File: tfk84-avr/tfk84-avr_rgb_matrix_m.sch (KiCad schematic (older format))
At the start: 42 parts

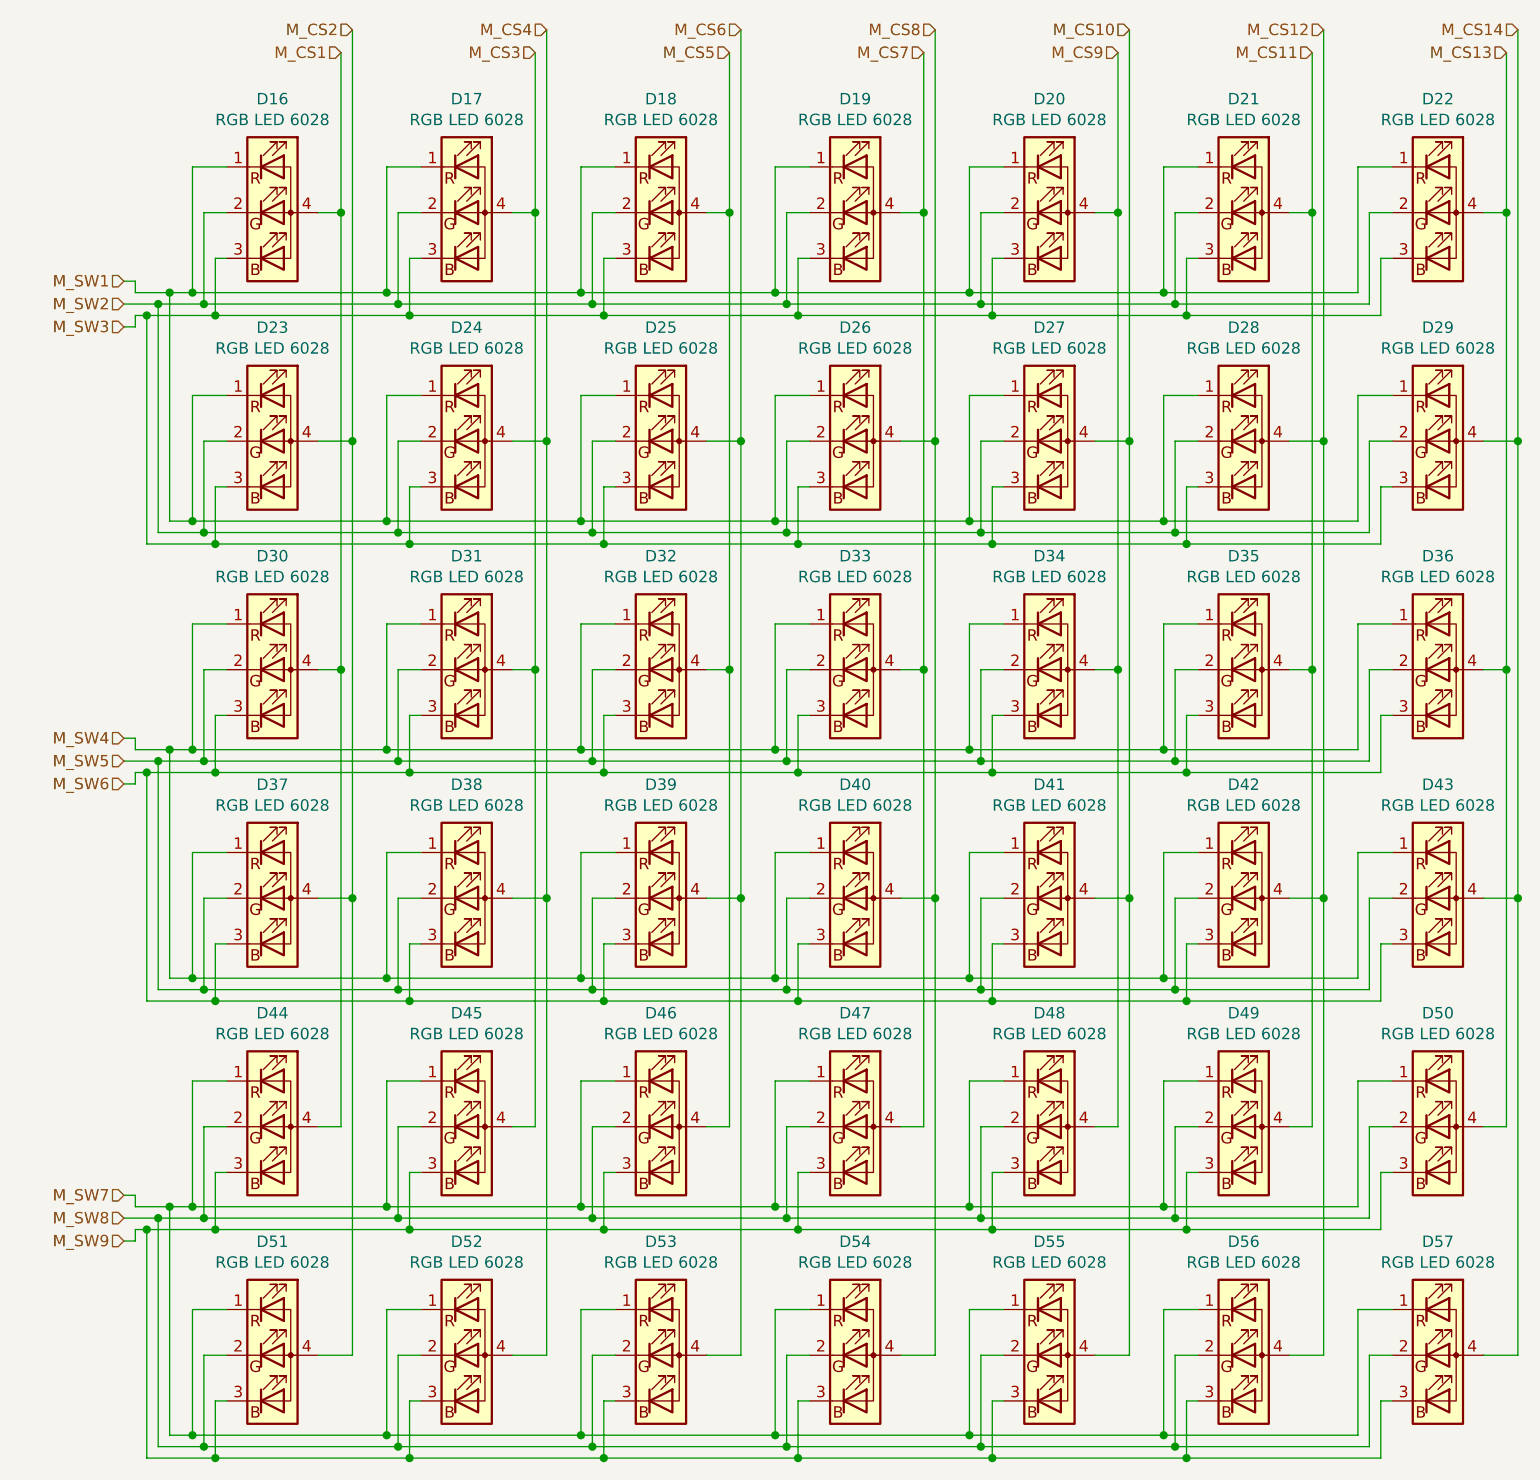
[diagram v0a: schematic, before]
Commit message: Begin PCB
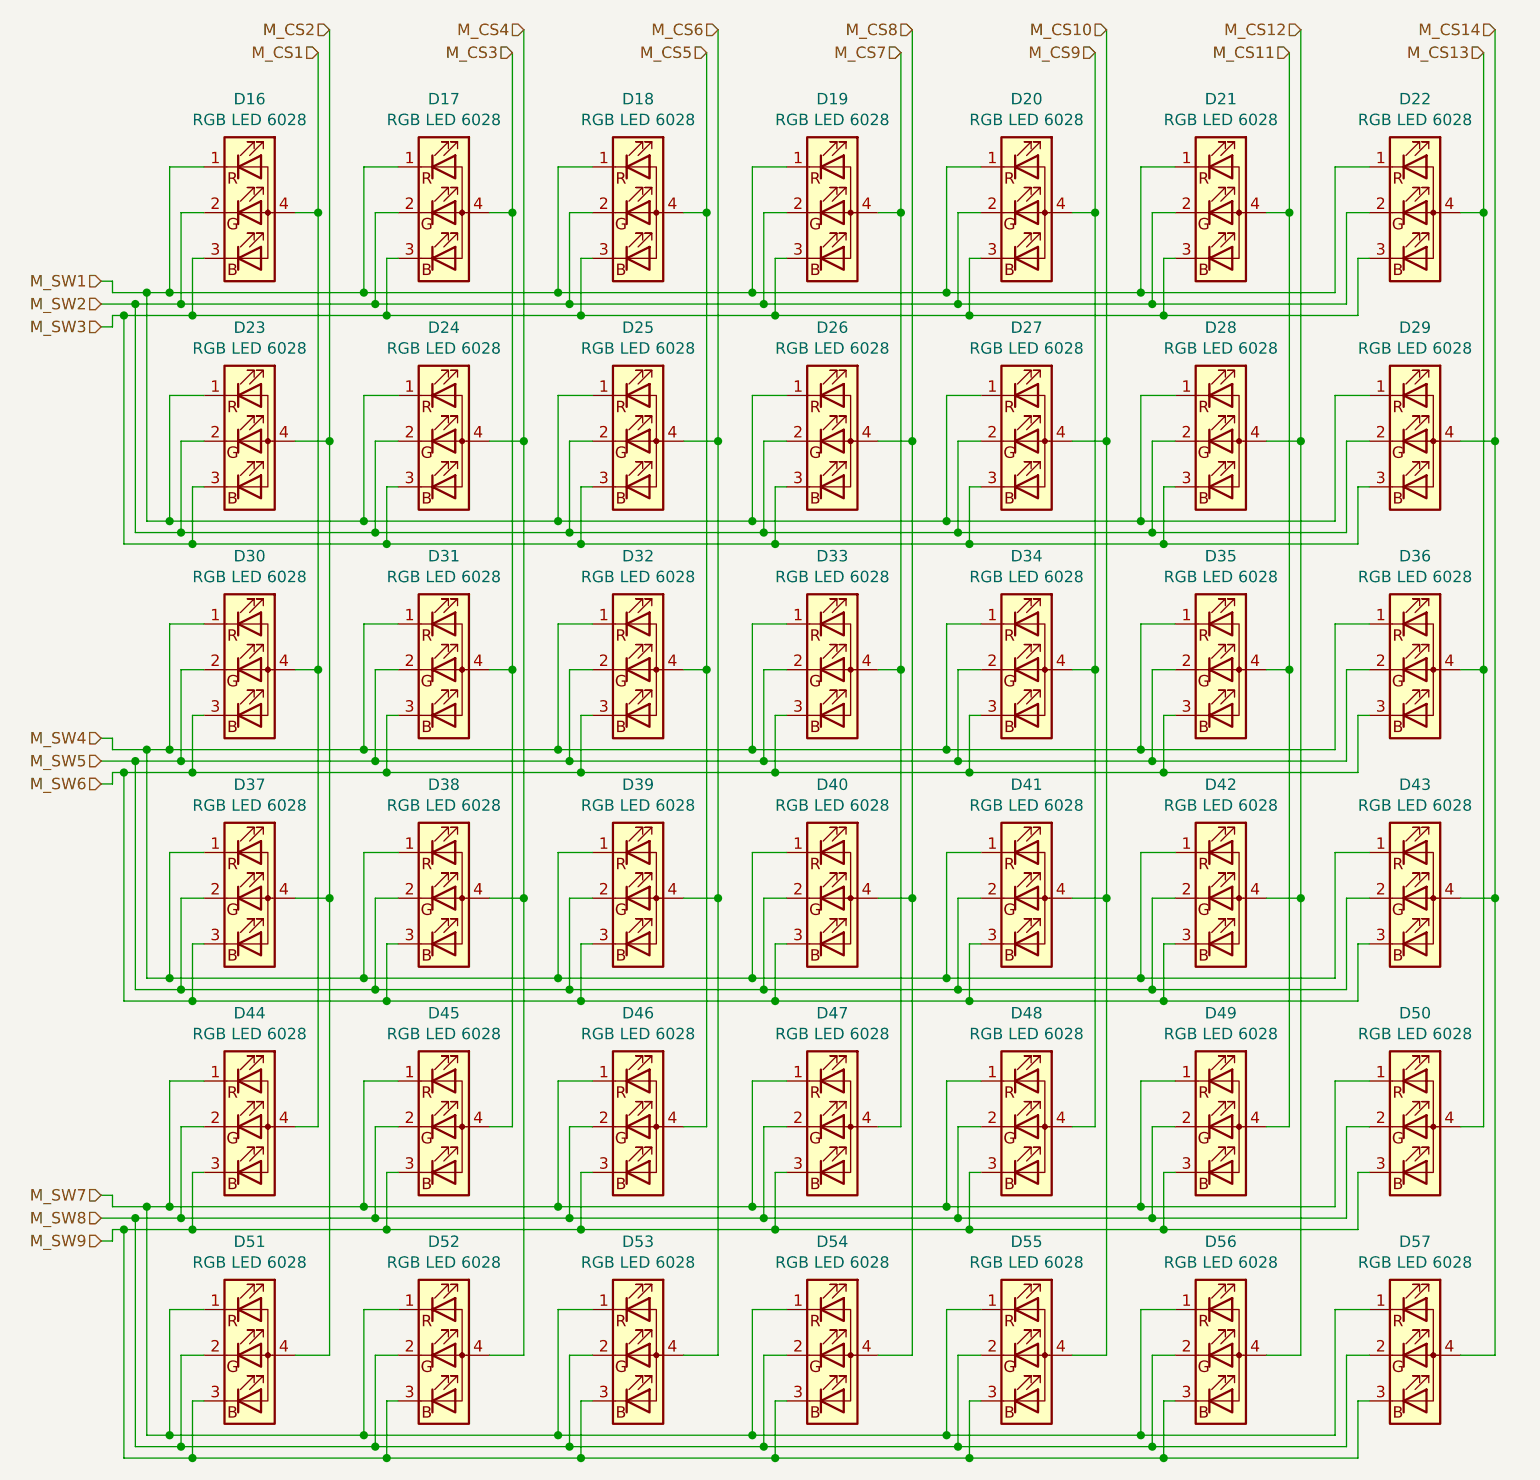
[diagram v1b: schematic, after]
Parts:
- D16, D17, D18, D19, D20, D21, D22, D23, D24, D25, D26, D27, D28, D29, D30, D31, D32, D33, D34, D35, D36, D37, D38, D39, D40, D41, D42, D43, D44, D45, D46, D47, D48, D49, D50, D51, D52, D53, D54, D55, D56, D57: footprint (none) -> random-keyboard-parts:RGB-6028
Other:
- moved on the sheet: D16, D17, D18, D19, D20, D21, D22, D23, D24, D25, D26, D27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
